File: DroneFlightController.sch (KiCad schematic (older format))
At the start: 1 part, among them U1 STM32H743VITx

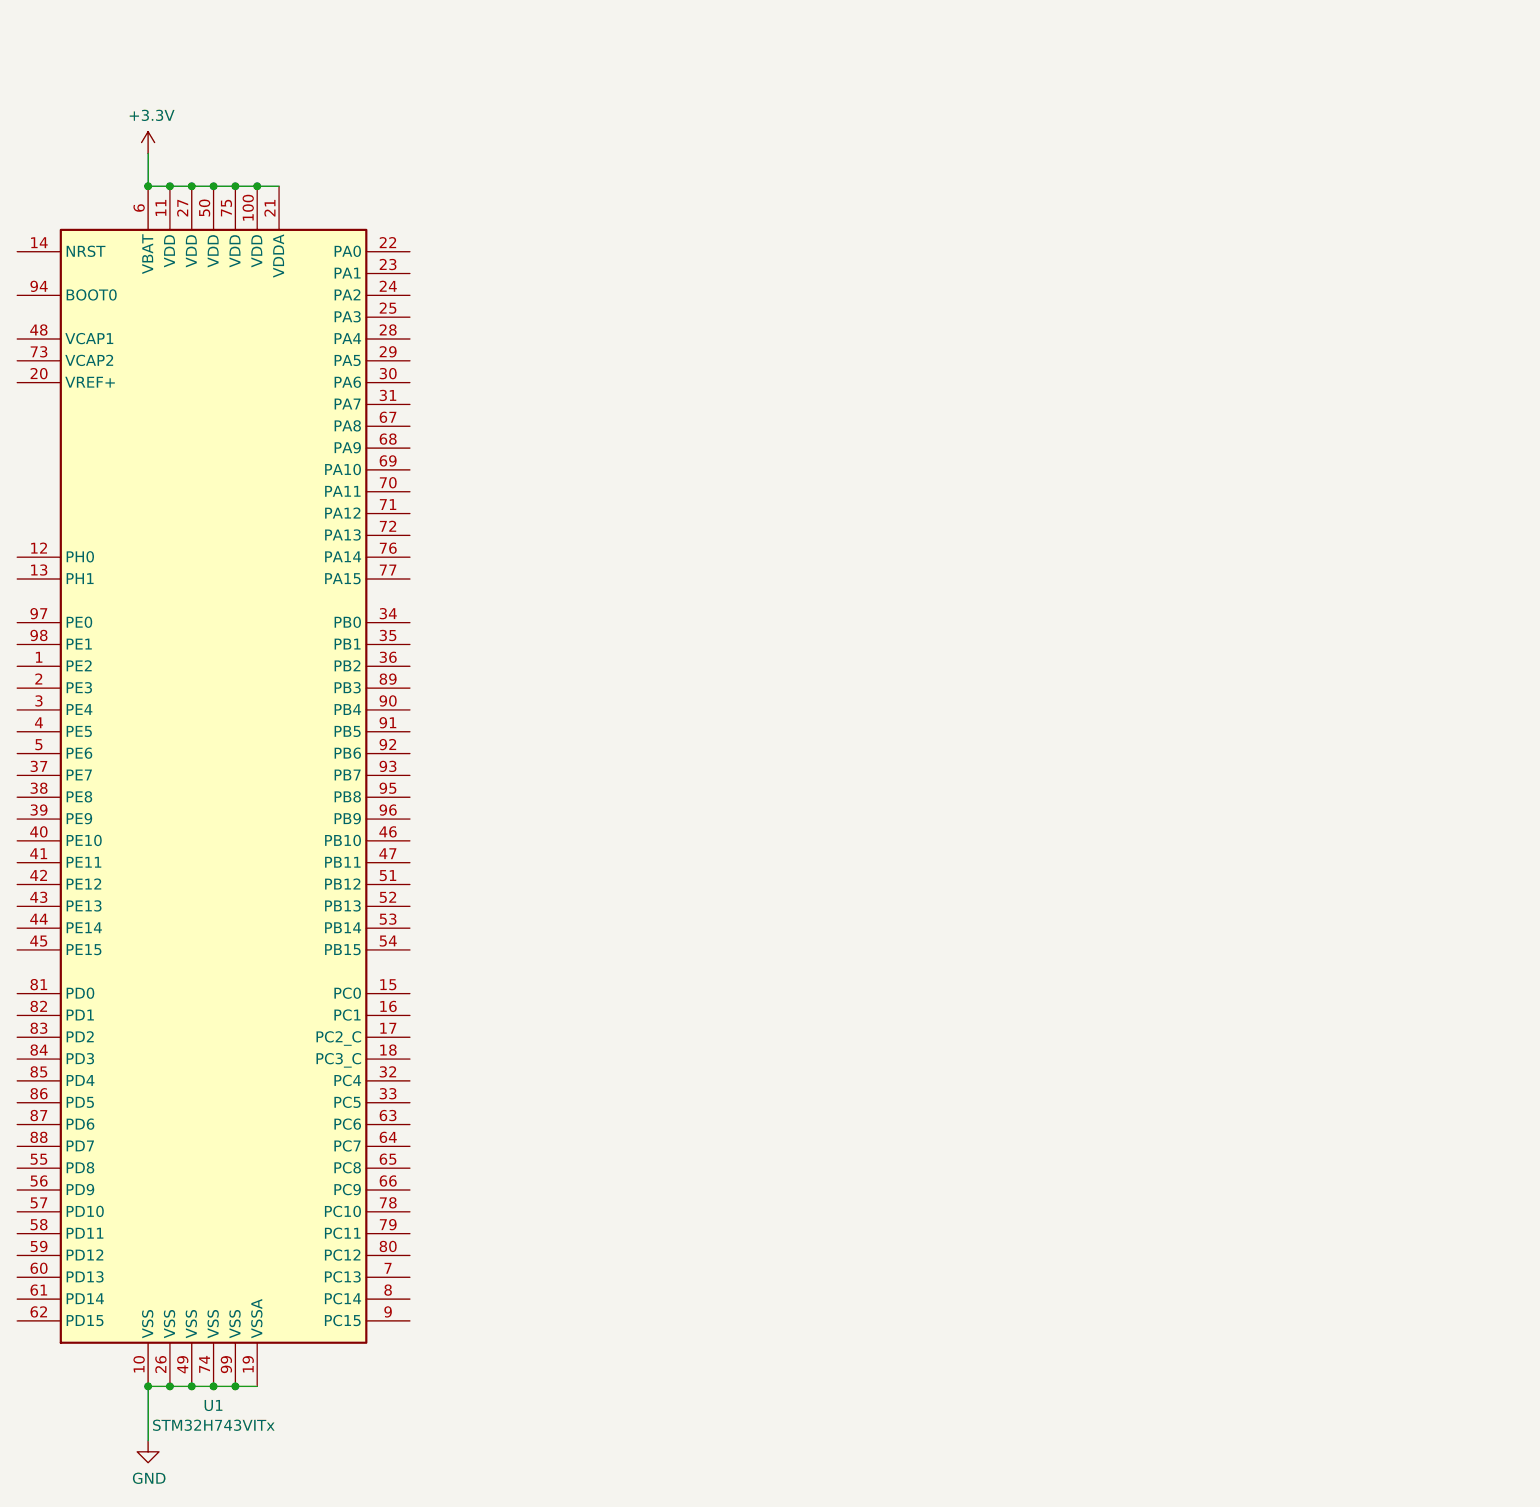
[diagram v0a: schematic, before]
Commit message: something started
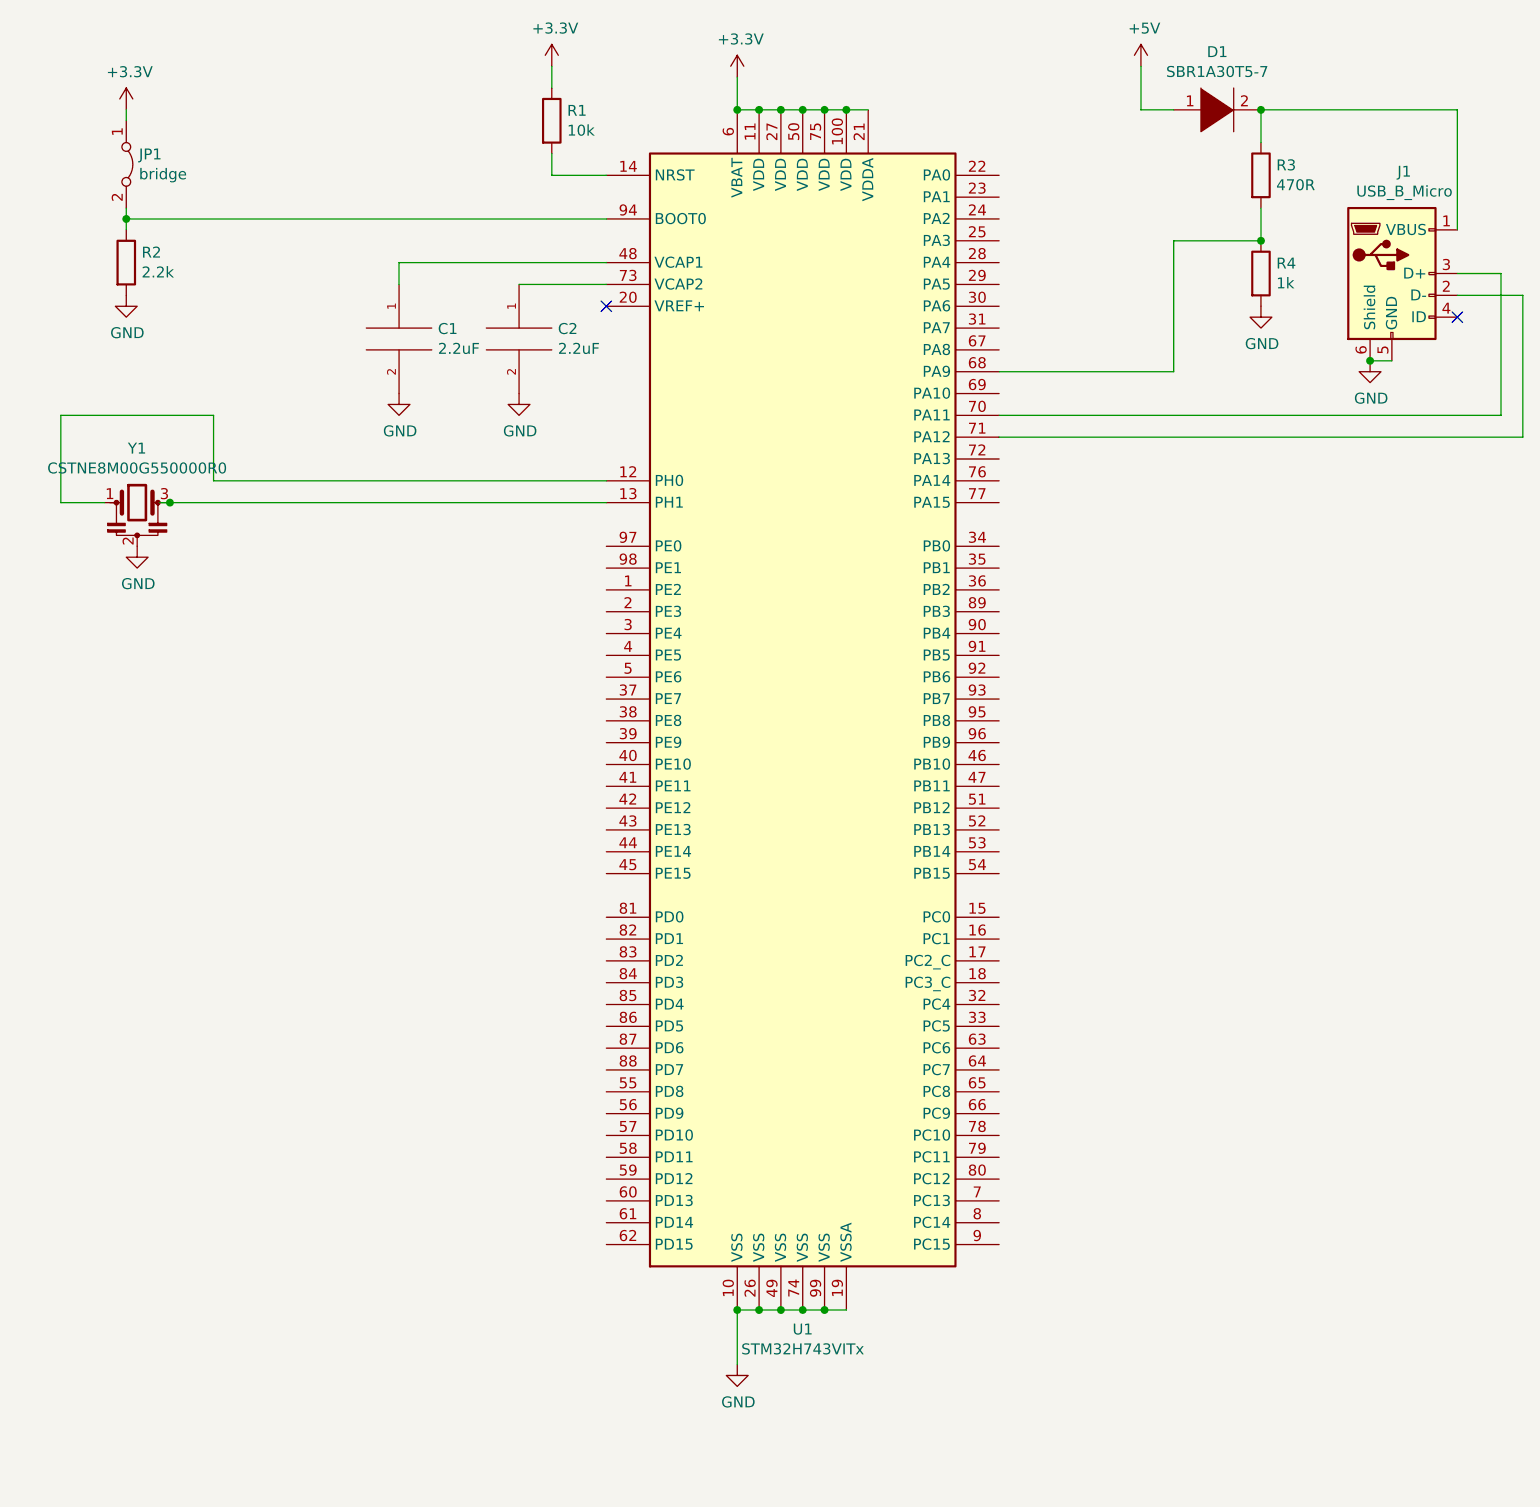
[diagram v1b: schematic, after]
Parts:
- added C1, C2: 2.2uF, symbol pspice:C
- added D1: SBR1A30T5-7, symbol pspice:DIODE
- added J1: USB_B_Micro, symbol Connector:USB_B_Micro
- added JP1: bridge, symbol Jumper:Jumper_2_Bridged
- added R1: 10k, symbol Device:R
- added R2: 2.2k, symbol Device:R
- added R3: 470R, symbol Device:R
- added R4: 1k, symbol Device:R
- added Y1: CSTNE8M00G550000R0, symbol Device:Resonator
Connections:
- net +3V3: now also JP1.1 (A), R1.1
- net GND: now also C1.2, C2.2, J1.5 (GND), J1.6 (Shield), R2.2, R4.2, Y1.2
- net at U1.12 (PH0): now also Y1.1
- net at U1.13 (PH1): now also Y1.3
- net at U1.14 (NRST): now also R1.2
- net at U1.48 (VCAP1): now also C1.1
- net at U1.68 (PA9): now also R3.2, R4.1
- net at U1.70 (PA11): now also J1.3 (D+)
- net at U1.71 (PA12): now also J1.2 (D-)
- net at U1.73 (VCAP2): now also C2.1
- net at U1.94 (BOOT0): now also JP1.2 (B), R2.1
- new net: D1.2 (A), J1.1 (VBUS), R3.1
- new net +5V: D1.1 (K)
- no-connect marks 0 -> 2
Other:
- moved on the sheet: U1
